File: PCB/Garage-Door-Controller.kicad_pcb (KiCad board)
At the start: 2 copper layers, 29.5 x 54 mm, 37 parts, among them J2 Conn_01x07_Pin, J3 Conn_01x07_Pin, J4 Screw_Terminal_01x02, J5 Screw_Terminal_01x02, SW1 TS-1088-AR02016, SW2 TS-1088-AR02016, SW3 PWR, U1 ESP32-C3-MINI-1, U2 AMS1117-3.3, U3 LTV-817S-TA1-C

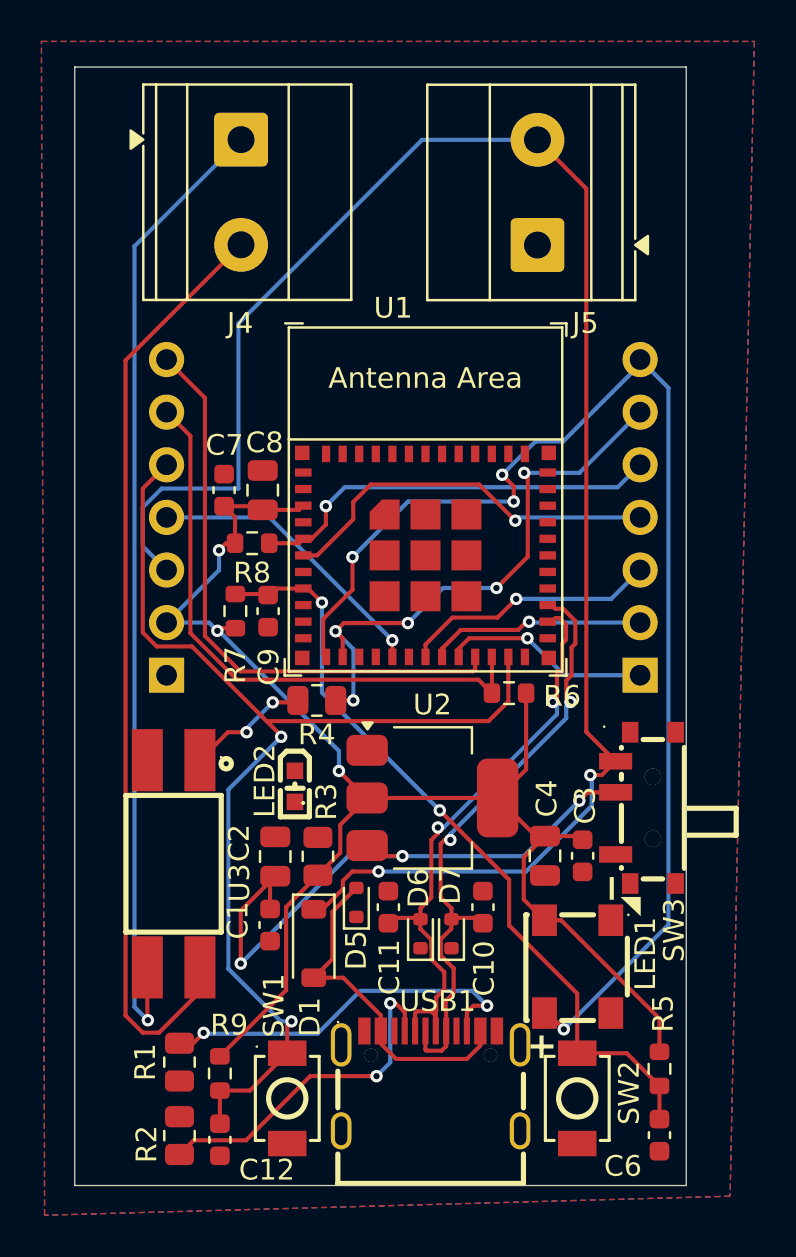
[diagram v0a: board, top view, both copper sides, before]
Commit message: Routed PCB
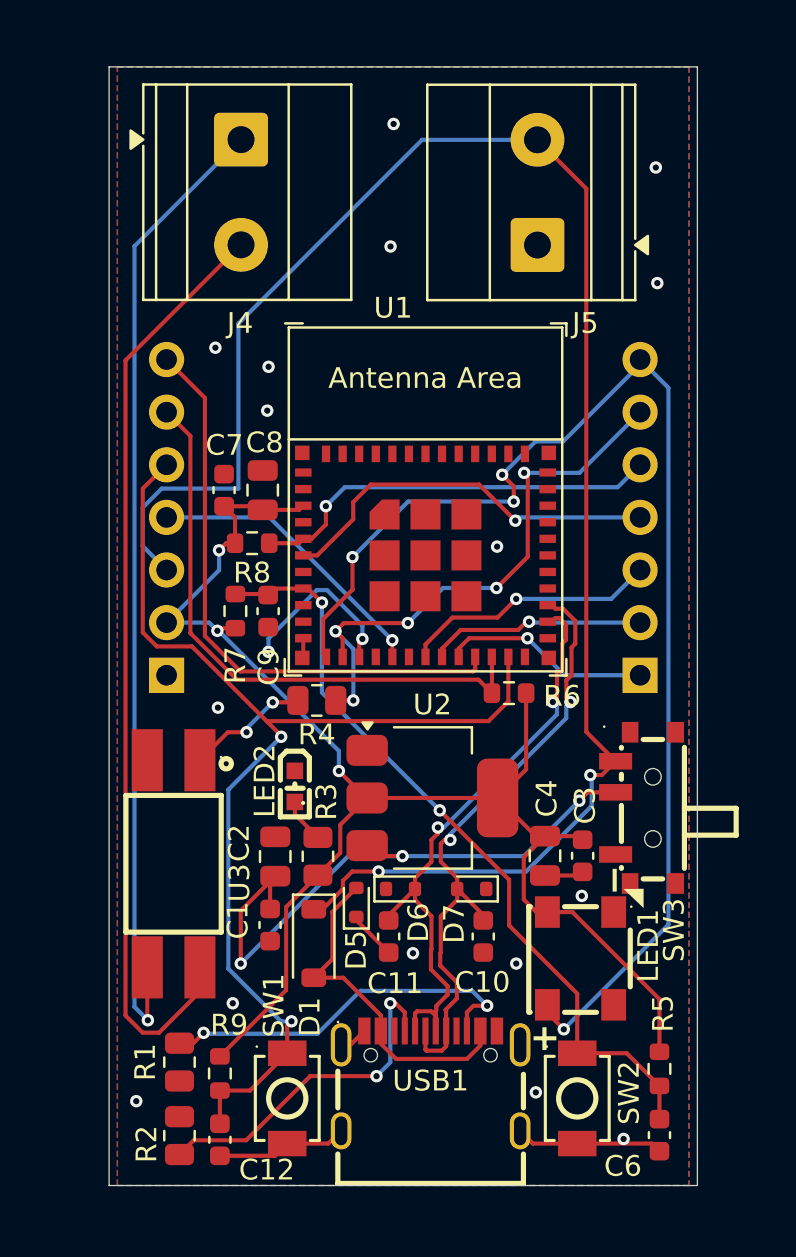
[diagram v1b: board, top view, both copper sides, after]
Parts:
- moved D7 2.37 mm to (35.3, 55.8), turned to 180 degrees
- moved D6 2.37 mm to (31.9, 55.8), turned to 0 degrees
- moved C10 1.42 mm to (35.9, 58.1), turned to -90 degrees
- moved C11 1.42 mm to (31.3, 58.1), turned to -90 degrees
- moved LED1 0.42 mm to (40.6, 59.1)
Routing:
- net GND: track 0.00 -> 28.5 mm, vias 0 -> 18
- net Net-(LED2-A): track 0.00 -> 2.17 mm
- net D +: track 29.8 -> 30.5 mm
- net D -: track 29.2 -> 29.9 mm
- net VCC_3V3: track 72.8 -> 73.4 mm
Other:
- board size 29.5 x 54 mm -> 28.4 x 54 mm
